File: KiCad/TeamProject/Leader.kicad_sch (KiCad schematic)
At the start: 9 parts, among them SW1 Reset, U1 PIC32MX170F256B

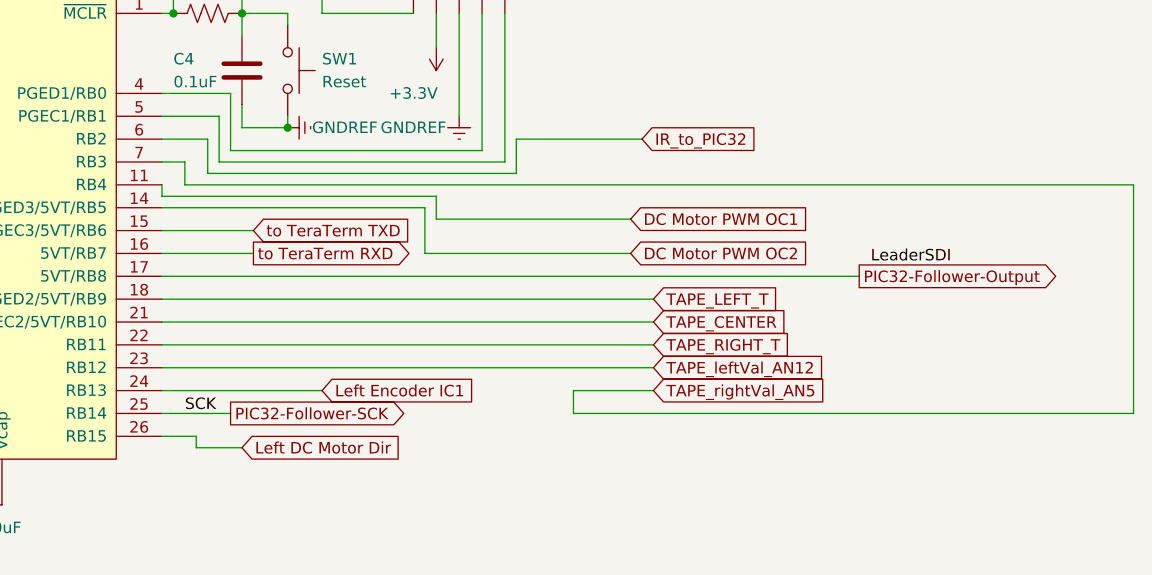
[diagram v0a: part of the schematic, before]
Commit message: Update connection for leader pic
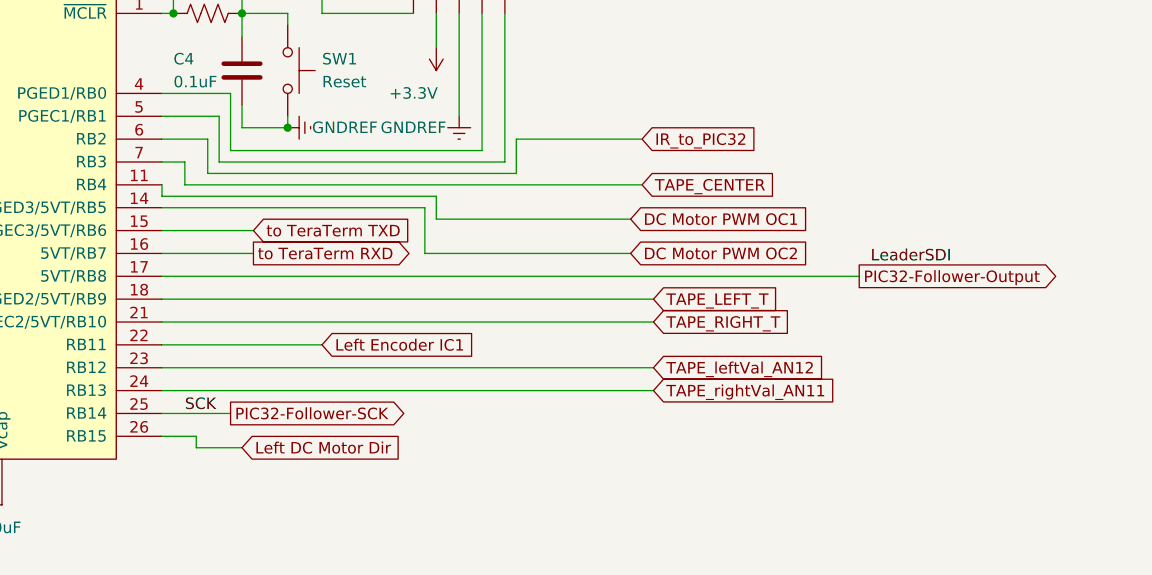
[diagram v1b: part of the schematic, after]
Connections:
- net TAPE_rightVal_AN5 is gone; now on net TAPE_CENTER: U1.7 (RB3)
- net Left Encoder IC1: now also U1.22 (RB11); no longer U1.24 (RB13)
- net TAPE_CENTER: no longer U1.21 (PGEC2/5VT/RB10)
- net TAPE_RIGHT_T: now also U1.21 (PGEC2/5VT/RB10); no longer U1.22 (RB11)
- new net TAPE_rightVal_AN11: U1.24 (RB13)
